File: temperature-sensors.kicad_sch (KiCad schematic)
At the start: 59 parts, among them J1 Conn_01x03, J2 USB_C_Receptacle_PowerOnly_6P, J3 Conn_01x02, J4 Conn_01x04, Q1 AO3401A, Q2 AO3401A, Q3 AO3401A, SW1 SW_Push, SW2 SW_SPST, U1 nRF52840-QFXX, U2 TP4057, U3 AMS1117-3.3, U5 SN74LVC1G00DCK, Y1 32MHz, Y2 32.768kHz

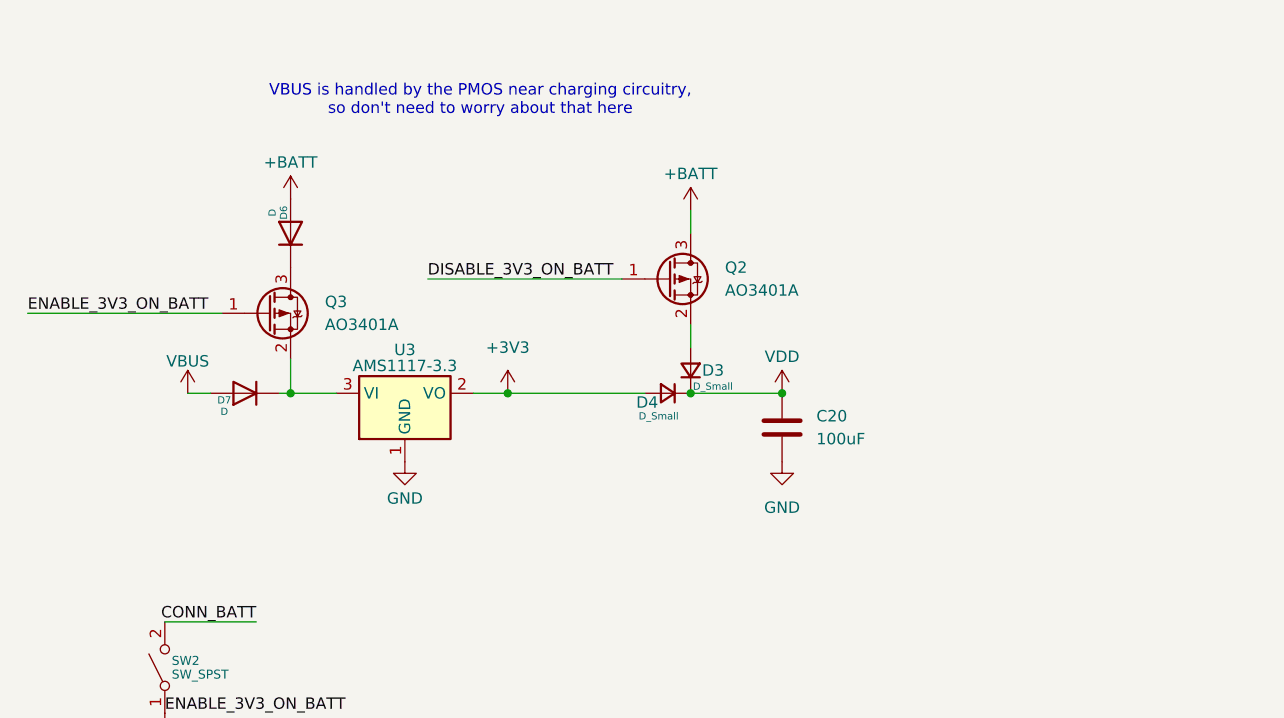
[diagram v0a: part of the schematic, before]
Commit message: aaaaaa
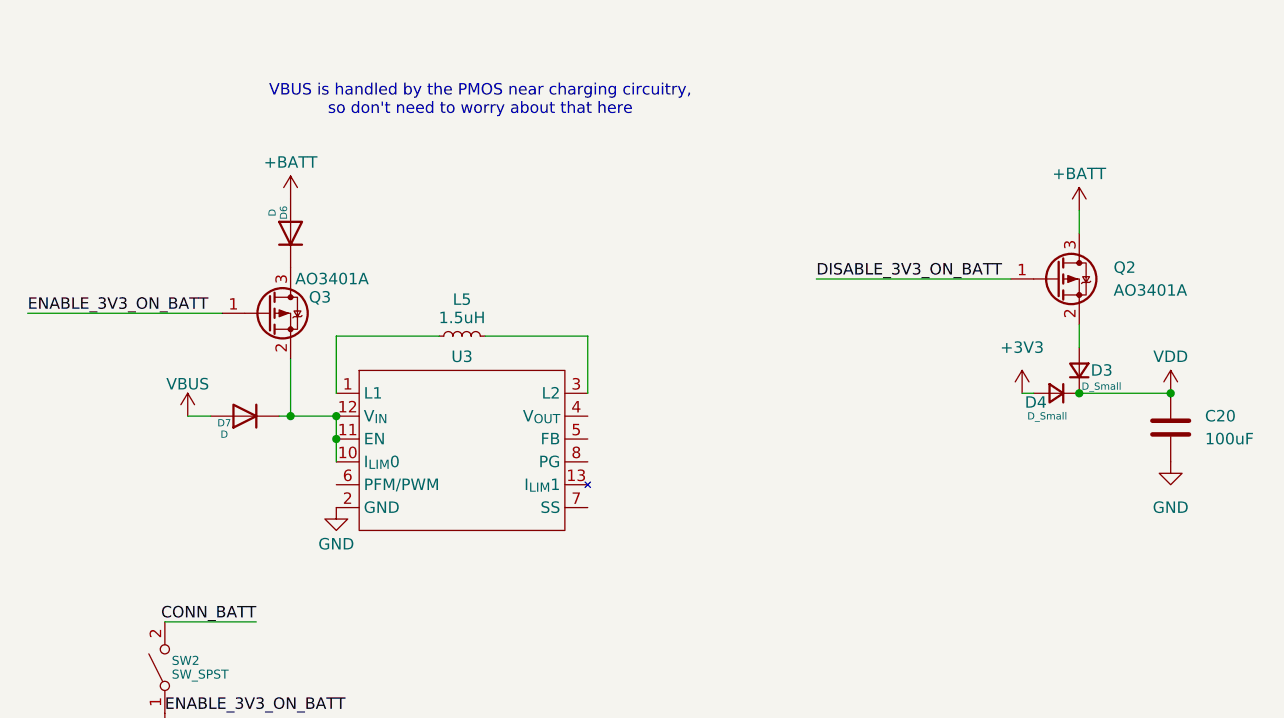
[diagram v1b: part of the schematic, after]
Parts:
- removed U3: AMS1117-3.3, Package_TO_SOT_SMD:SOT-223-3_TabPin2, symbol KiCad:AMS1117-3.3
- added L5: 1.5uH, symbol KiCad:L_Small
- added U3: (no value), temp-sensors:TPS63051-QFN-12-HotRod, symbol temp-sensors:TPS63051
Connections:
- net GND: now also U3.2 (GND)
- net at D7.1 (K), Q3.2 (S): now also U3.10 (I_{LIM}0), U3.11 (EN), U3.12 (V_{IN})
- new net: L5.1, U3.1 (L1)
- new net: L5.2, U3.3 (L2)
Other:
- moved on the sheet: C20, D3, D4, D7, Q2
